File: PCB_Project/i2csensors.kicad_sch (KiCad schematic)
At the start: 25 parts, among them J3 Motor_Connector

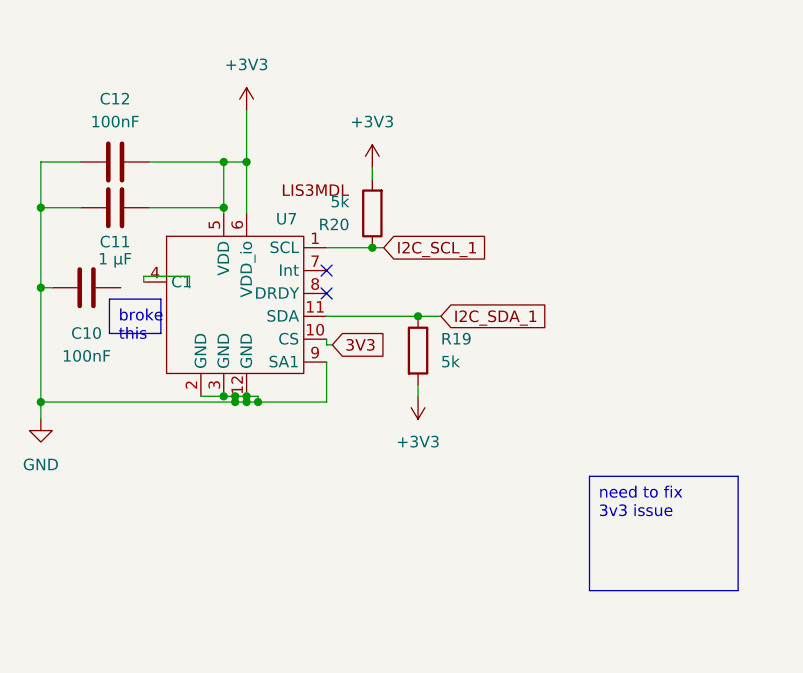
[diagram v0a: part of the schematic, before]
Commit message: working on root sch
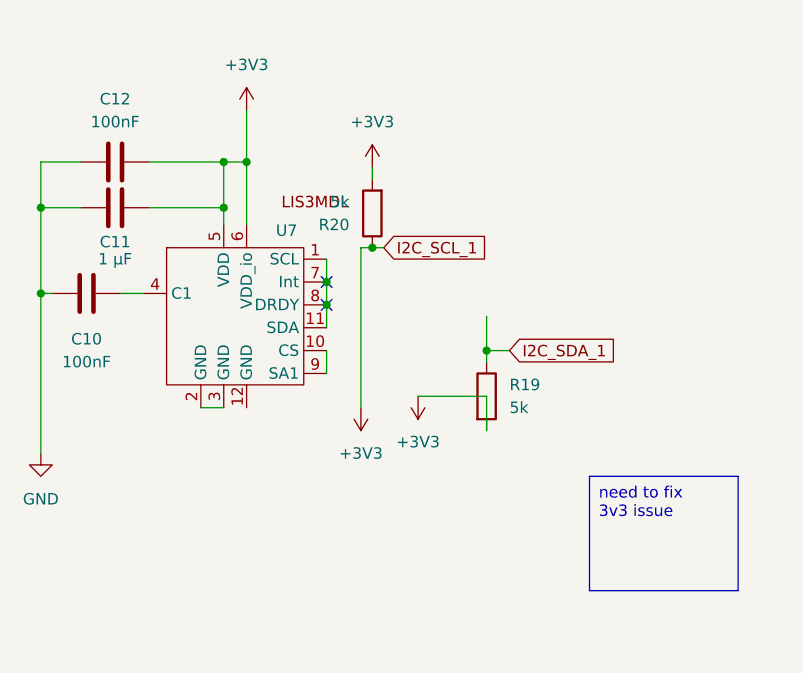
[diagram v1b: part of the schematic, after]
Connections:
- net +3V3: now also R20.1, R6.2, U11.1 (SCL)
- net 3V3: no longer U7.10 (CS)
- net GND: no longer U7.12 (GND), U7.2 (GND), U7.3 (GND), U7.9 (SA1)
- net I2C_SDA_1: no longer U7.11 (SDA)
- net at C10.1: now also U7.4 (C1)
- net at U7.7 (Int): now also U7.1 (SCL), U7.11 (SDA), U7.8 (DRDY)
- removed net I2C_SCL_1: R20.1, R6.2, U11.1 (SCL), U7.1 (SCL)
- new net: U7.10 (CS), U7.9 (SA1)
- new net: U7.2 (GND), U7.3 (GND)
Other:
- moved on the sheet: C10, R19, U7

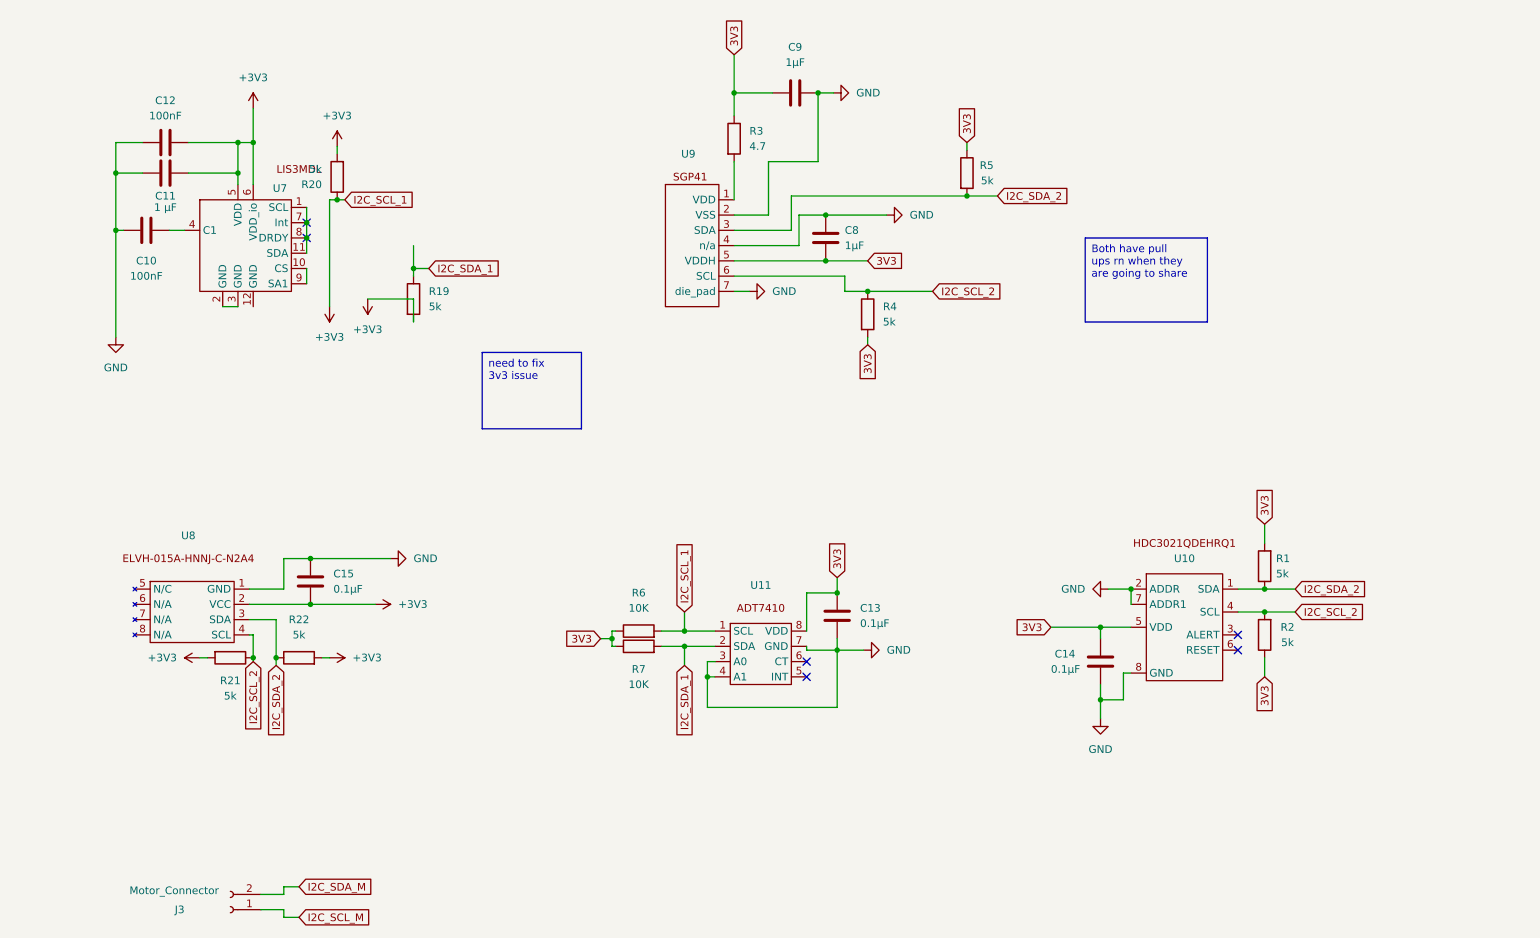
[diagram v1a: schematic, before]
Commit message: work baby
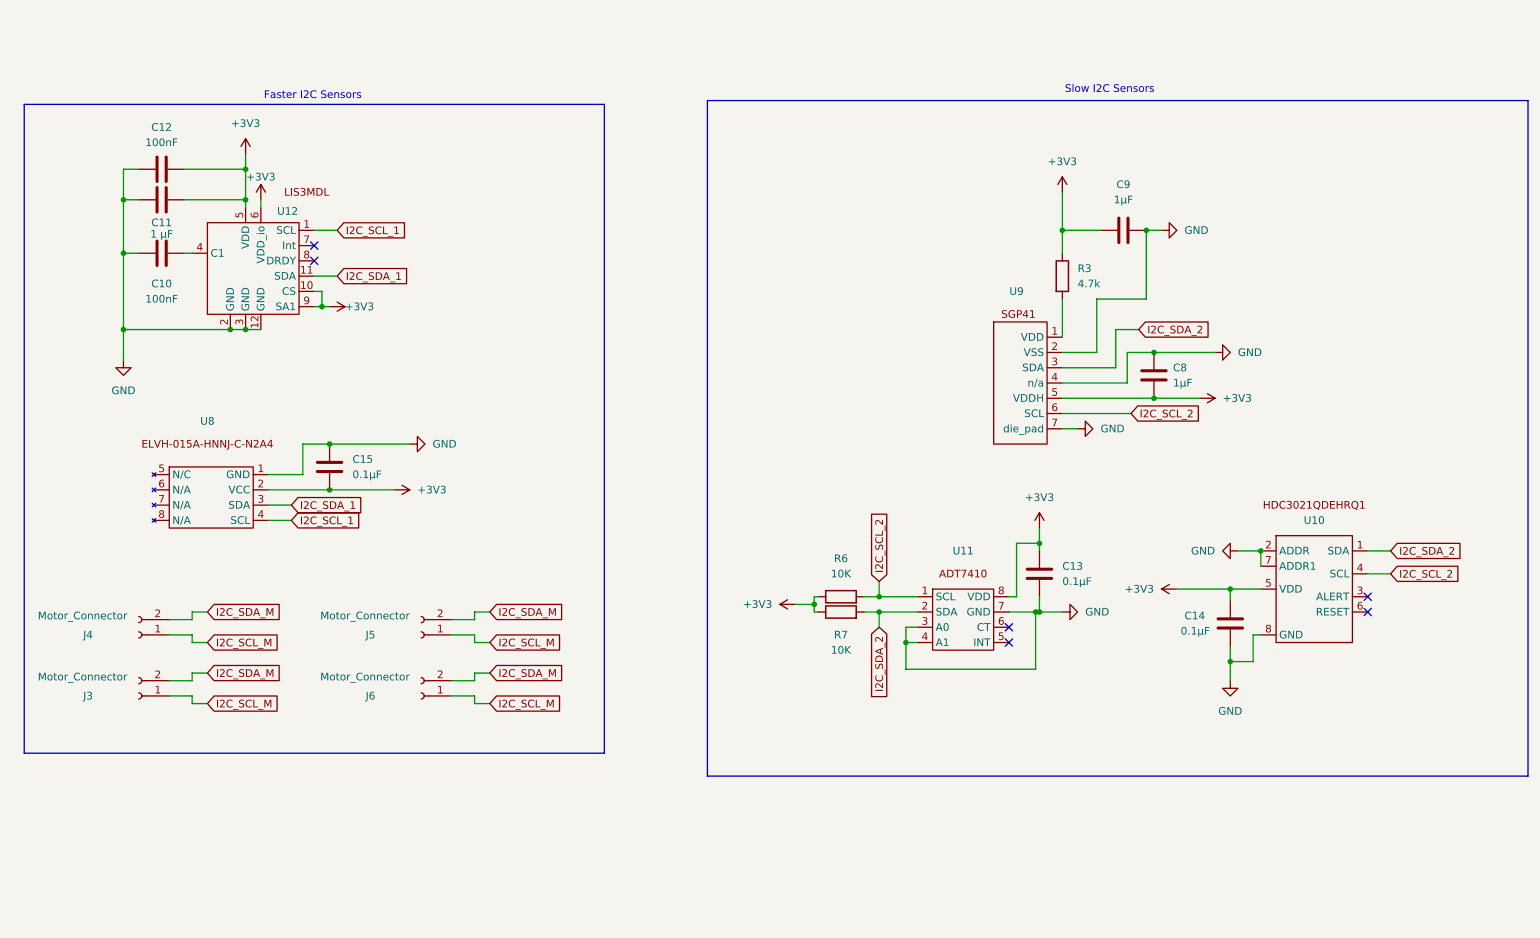
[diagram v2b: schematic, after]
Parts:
- removed R1, R19, R2, R20, R21, R22, R4, R5: 5k, symbol Device:R
- removed U7: ~, symbol sensors:LIS3MDL
- added J4, J5, J6: Motor_Connector, symbol Connector:Conn_01x02_Socket
- added U12: ~, symbol sensors:LIS3MDL
- C10, C12: footprint (none) -> Capacitor_SMD:C_0603_1608Metric
- C11, C13, C14, C15, C8, C9: footprint (none) -> Capacitor_SMD:C_0402_1005Metric
- R3: value 4.7 -> 4.7k; footprint (none) -> Resistor_SMD:R_0603_1608Metric
- R6, R7: footprint (none) -> Resistor_SMD:R_0603_1608Metric
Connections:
- net 3V3 is gone; now on net +3V3: C13.1, C14.1, C8.2, C9.1, R3.1, R6.1, R7.1, U10.5 (VDD), U11.8 (VDD), U9.5 (VDDH)
- net +3V3: now also U12.10 (CS), U12.5 (VDD), U12.6 (VDD_io), U12.9 (SA1); no longer R6.2, U11.1 (SCL)
- net GND: now also U12.12 (GND), U12.2 (GND), U12.3 (GND)
- net I2C_SCL_2: now also R6.2, U11.1 (SCL); no longer U8.4 (SCL)
- net I2C_SCL_M: now also J4.1 (Pin_1), J5.1 (Pin_1), J6.1 (Pin_1)
- net I2C_SDA_1: now also U8.3 (SDA), U12.11 (SDA); no longer R7.2, U11.2 (SDA)
- net I2C_SDA_2: now also R7.2, U11.2 (SDA); no longer U8.3 (SDA)
- net I2C_SDA_M: now also J4.2 (Pin_2), J5.2 (Pin_2), J6.2 (Pin_2)
- net at C10.1: now also U12.4 (C1)
- new net I2C_SCL_1: U12.1 (SCL), U8.4 (SCL)
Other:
- note added: "Faster I2C Sensors"
- note added: "Slow I2C Sensors"
- moved on the sheet: C10, C11, C12, C13, C14, C15, C8, C9, J3, R3, R6, R7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

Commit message: 2 footprints left then can design
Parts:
- C10, C12: footprint Capacitor_SMD:C_0603_1608Metric -> Capacitor_SMD:C_0402_1005Metric
- J3, J4, J5, J6: footprint (none) -> Connector_JST:JST_PH_B2B-PH-K_1x02_P2.00mm_Vertical
- R3, R6, R7: footprint Resistor_SMD:R_0603_1608Metric -> Resistor_SMD:R_0402_1005Metric
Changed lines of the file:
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@@
 			)
 		)
-		(property "Footprint" ""
+		(property "Footprint" "Connector_JST:JST_PH_B2B-PH-K_1x02_P2.00mm_Vertical"
 			(at 48.26 132.08 0)
 			(effects
@@
 			)
 		)
-		(property "Footprint" "Capacitor_SMD:C_0603_1608Metric"
+		(property "Footprint" "Capacitor_SMD:C_0402_1005Metric"
 			(at 48.26 59.3852 0)
 			(effects
@@
 			)
 		)
-		(property "Footprint" "Capacitor_SMD:C_0603_1608Metric"
+		(property "Footprint" "Capacitor_SMD:C_0402_1005Metric"
 			(at 48.26 45.4152 0)
 			(effects
@@
 			)
 		)
-		(property "Footprint" ""
+		(property "Footprint" "Connector_JST:JST_PH_B2B-PH-K_1x02_P2.00mm_Vertical"
 			(at 95.25 132.08 0)
 			(effects
@@
 			)
 		)
-		(property "Footprint" ""
+		(property "Footprint" "Connector_JST:JST_PH_B2B-PH-K_1x02_P2.00mm_Vertical"
 			(at 48.26 121.92 0)
 			(effects
@@
 			)
 		)
-		(property "Footprint" "Resistor_SMD:R_0603_1608Metric"
+		(property "Footprint" "Resistor_SMD:R_0402_1005Metric"
 			(at 165.1 117.348 90)
 			(effects
@@
 			)
 		)
-		(property "Footprint" ""
+		(property "Footprint" "Connector_JST:JST_PH_B2B-PH-K_1x02_P2.00mm_Vertical"
 			(at 95.25 121.92 0)
 			(effects
@@
 			)
 		)
-		(property "Footprint" "Resistor_SMD:R_0603_1608Metric"
+		(property "Footprint" "Resistor_SMD:R_0402_1005Metric"
 			(at 165.1 119.888 90)
 			(effects
@@
 			)
 		)
-		(property "Footprint" "Resistor_SMD:R_0603_1608Metric"
+		(property "Footprint" "Resistor_SMD:R_0402_1005Metric"
 			(at 200.152 62.23 90)
 			(effects

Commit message: pcb work
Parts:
- U10: footprint (none) -> Sensor:WSON8_DEH_TEX
- U11: footprint (none) -> Sensor:SOIC127P600X175-8N_ADT7410TRZ-REEL
- U12: footprint (none) -> Package_LGA:LGA-12_2x2mm_P0.5mm
- U9: footprint (none) -> Sensor:XDCR_SGP41-D-R4
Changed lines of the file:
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@@
 			)
 		)
-		(property "Footprint" ""
+		(property "Footprint" "Package_LGA:LGA-12_2x2mm_P0.5mm"
 			(at 69.85 69.85 0)
 			(effects
@@
 			)
 		)
-		(property "Footprint" ""
+		(property "Footprint" "Sensor:SOIC127P600X175-8N_ADT7410TRZ-REEL"
 			(at 185.42 124.46 0)
 			(effects
@@
 			)
 		)
-		(property "Footprint" ""
+		(property "Footprint" "Sensor:XDCR_SGP41-D-R4"
 			(at 199.39 74.93 0)
 			(effects
@@
 			)
 		)
-		(property "Footprint" ""
+		(property "Footprint" "Sensor:WSON8_DEH_TEX"
 			(at 245.11 114.3 0)
 			(effects
